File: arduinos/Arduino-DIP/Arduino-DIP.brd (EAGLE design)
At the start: 23.5 x 57.3 mm, 16 parts, among them IC1 ATMEGA 328, IC2 MCP1702-33, X1 16 MHz

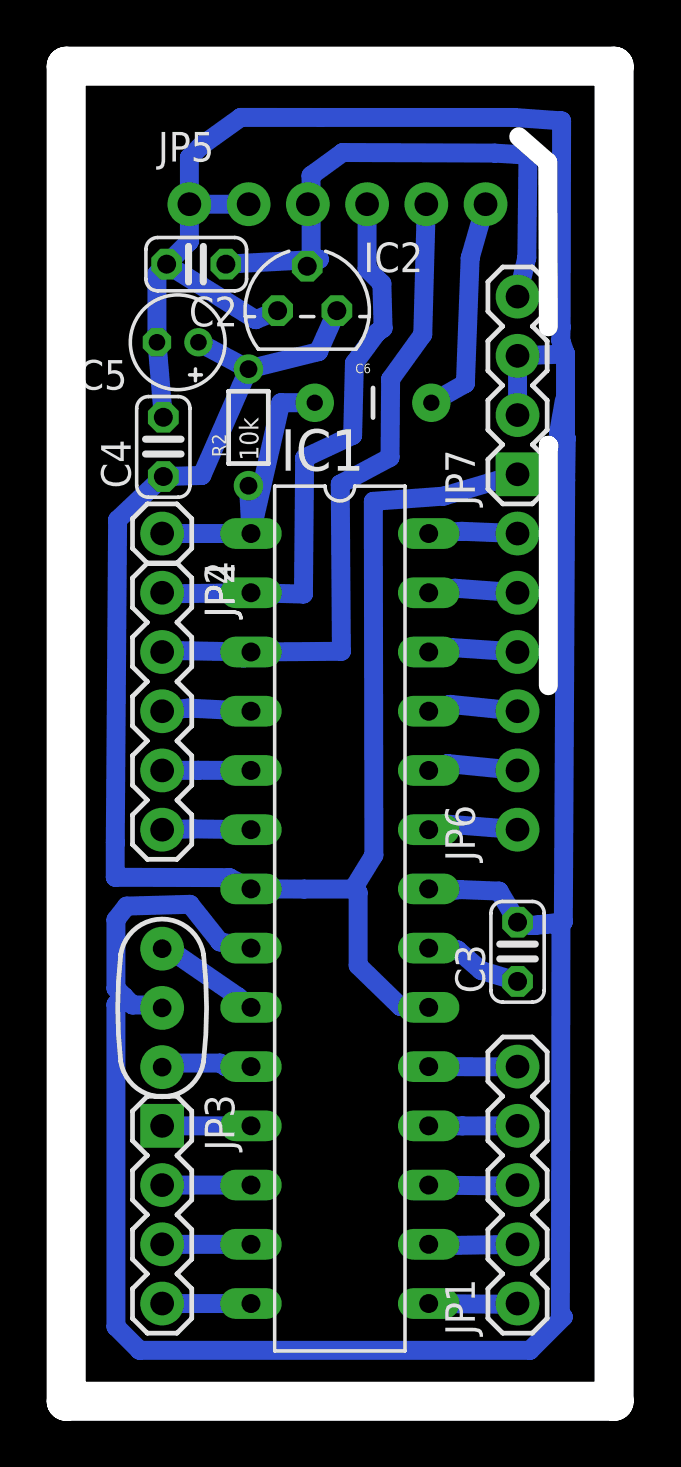
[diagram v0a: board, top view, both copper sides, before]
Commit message: much commit, so wow
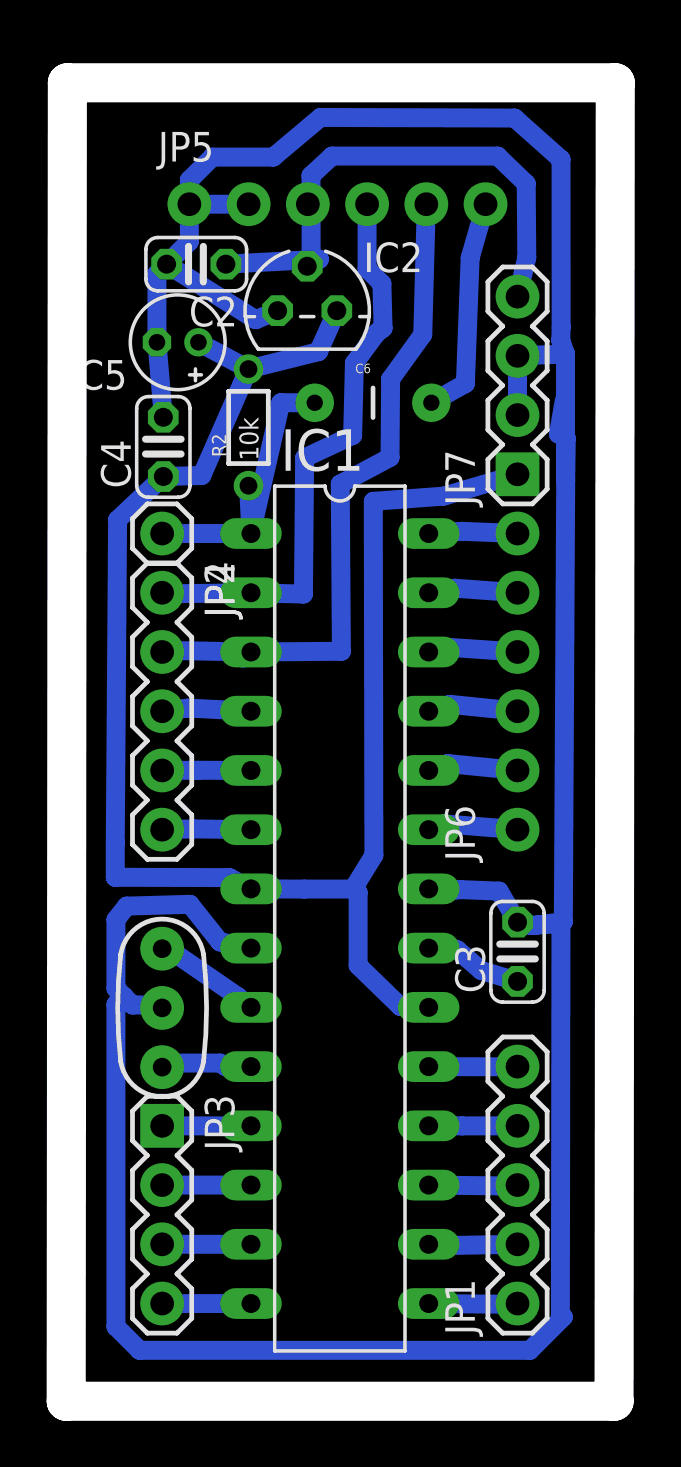
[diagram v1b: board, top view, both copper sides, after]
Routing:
- net GND: track 150.5 -> 149.0 mm
- net PWR: track 24.3 -> 23.5 mm
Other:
- board size 23.5 x 57.3 mm -> 23.5 x 56.5 mm
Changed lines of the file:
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@@
 <layer number="21" name="tPlace" color="7" fill="1" visible="yes" active="yes"/>
 <layer number="22" name="bPlace" color="7" fill="1" visible="yes" active="yes"/>
-<layer number="23" name="tOrigins" color="15" fill="1" visible="yes" active="yes"/>
-<layer number="24" name="bOrigins" color="15" fill="1" visible="yes" active="yes"/>
+<layer number="23" name="tOrigins" color="15" fill="1" visible="no" active="yes"/>
+<layer number="24" name="bOrigins" color="15" fill="1" visible="no" active="yes"/>
 <layer number="25" name="tNames" color="7" fill="1" visible="no" active="yes"/>
 <layer number="26" name="bNames" color="7" fill="1" visible="no" active="yes"/>
@@
 <layer number="112" name="tSilk" color="7" fill="1" visible="yes" active="yes"/>
 <layer number="113" name="IDFDebug" color="4" fill="1" visible="yes" active="yes"/>
-<layer number="114" name="roland_bottom_32" color="11" fill="1" visible="yes" active="yes"/>
+<layer number="114" name="roland_bottom_32" color="11" fill="1" visible="no" active="yes"/>
 <layer number="116" name="Patch_BOT" color="9" fill="4" visible="yes" active="yes"/>
 <layer number="121" name="_tsilk" color="7" fill="1" visible="yes" active="yes"/>
@@
 A0</text>
 <wire x1="0" y1="0" x2="23.495" y2="0" width="1.6764" layer="20"/>
-<wire x1="23.495" y1="0" x2="23.495" y2="57.2516" width="1.6764" layer="20"/>
-<wire x1="23.495" y1="57.2516" x2="0" y2="57.2516" width="1.6764" layer="20"/>
-<wire x1="0" y1="57.2516" x2="0" y2="0" width="1.6764" layer="20"/>
+<wire x1="23.495" y1="0" x2="23.5458" y2="56.5404" width="1.6764" layer="20"/>
+<wire x1="23.5458" y1="56.5404" x2="0.0508" y2="56.5404" width="1.6764" layer="20"/>
+<wire x1="0.0508" y1="56.5404" x2="0" y2="0" width="1.6764" layer="20"/>
 <wire x1="14.3002" y1="2.9718" x2="9.271" y2="2.9718" width="0.8128" layer="114"/>
-<wire x1="19.4056" y1="54.229" x2="20.6502" y2="53.1368" width="0.8128" layer="46"/>
-<wire x1="20.6502" y1="53.1368" x2="20.6756" y2="46.0756" width="0.8128" layer="46"/>
-<wire x1="20.701" y1="40.9702" x2="20.6756" y2="40.9956" width="0.8128" layer="46"/>
-<wire x1="20.6756" y1="40.9956" x2="20.6756" y2="30.6832" width="0.8128" layer="46"/>
+<wire x1="19.4056" y1="54.229" x2="20.6502" y2="53.1368" width="0.8128" layer="114"/>
+<wire x1="20.6502" y1="53.1368" x2="20.6756" y2="46.0756" width="0.8128" layer="114"/>
+<wire x1="20.701" y1="40.9702" x2="20.6756" y2="40.9956" width="0.8128" layer="114"/>
+<wire x1="20.6756" y1="40.9956" x2="20.6756" y2="30.6832" width="0.8128" layer="114"/>
 </plain>
 <attributes>
@@
 <wire x1="19.44059375" y1="20.4738" x2="19.3548" y2="20.5440125" width="0.8128" layer="16"/>
 <wire x1="21.2174" y1="20.493" x2="19.9524" y2="20.3992" width="0.8128" layer="16"/>
-<wire x1="21.2448" y1="54.907" x2="19.2048" y2="55.0532" width="0.8128" layer="16"/>
-<wire x1="19.2048" y1="55.0532" x2="10.9048" y2="55.0532" width="0.8128" layer="16"/>
-<wire x1="10.9048" y1="55.0532" x2="7.4856" y2="55.0548" width="0.8128" layer="16"/>
-<wire x1="7.4856" y1="55.0548" x2="5.784" y2="53.835428125" width="0.8128" layer="16"/>
-<wire x1="21.2448" y1="54.907" x2="21.225290625" y2="46.05624375" width="0.8128" layer="16"/>
+<wire x1="21.2194" y1="53.256" x2="19.2302" y2="55.0278" width="0.8128" layer="16"/>
+<wire x1="19.2302" y1="55.0278" x2="10.9048" y2="55.0532" width="0.8128" layer="16"/>
+<wire x1="10.9048" y1="55.0532" x2="8.8826" y2="53.353" width="0.8128" layer="16"/>
+<wire x1="8.8826" y1="53.353" x2="6.2666" y2="53.352828125" width="0.8128" layer="16"/>
+<wire x1="21.2194" y1="53.256" x2="21.225290625" y2="46.05624375" width="0.8128" layer="16"/>
 <wire x1="21.319" y1="20.561" x2="21.4206" y2="39.497" width="0.8128" layer="16"/>
 <wire x1="21.4206" y1="39.497" x2="21.446" y2="41.292" width="0.8128" layer="16"/>
@@
 <contactref element="JP5" pad="1"/>
 <contactref element="JP5" pad="2"/>
-<wire x1="5.2832" y1="51.3334" x2="5.2832" y2="53.334628125" width="0.8128" layer="16"/>
-<wire x1="5.2832" y1="53.334628125" x2="5.784" y2="53.835428125" width="0.8128" layer="16"/>
+<wire x1="5.2832" y1="51.3334" x2="5.2832" y2="52.369428125" width="0.8128" layer="16"/>
+<wire x1="5.2832" y1="52.369428125" x2="6.2666" y2="53.352828125" width="0.8128" layer="16"/>
 <wire x1="7.8232" y1="51.3334" x2="5.2832" y2="51.3334" width="0.8128" layer="16"/>
 <wire x1="5.2832" y1="51.3334" x2="5.2832" y2="49.738075" width="0.8128" layer="16"/>
@@
 <contactref element="IC2" pad="2"/>
 <contactref element="C2" pad="1"/>
-<wire x1="19.8032" y1="53.4358" x2="18.3746" y2="53.5246" width="0.8128" layer="16"/>
-<wire x1="18.3746" y1="53.5246" x2="11.8588" y2="53.55" width="0.8128" layer="16"/>
-<wire x1="11.8588" y1="53.55" x2="10.4984" y2="52.561" width="0.8128" layer="16"/>
+<wire x1="19.727" y1="52.2166" x2="18.5016" y2="53.3976" width="0.8128" layer="16"/>
+<wire x1="18.5016" y1="53.3976" x2="11.4016" y2="53.3976" width="0.8128" layer="16"/>
+<wire x1="11.4016" y1="53.3976" x2="10.4984" y2="52.561" width="0.8128" layer="16"/>
 <wire x1="10.4984" y1="52.561" x2="10.5048" y2="51.341028125" width="0.8128" layer="16"/>
 <wire x1="10.858109375" y1="48.971971875" x2="10.3359875" y2="48.6730875" width="0.8128" layer="16"/>
-<wire x1="19.7524" y1="49.0372" x2="19.8032" y2="53.4358" width="0.8128" layer="16"/>
+<wire x1="19.7524" y1="49.0372" x2="19.727" y2="52.2166" width="0.8128" layer="16"/>
 <wire x1="6.846940625" y1="48.761815625" x2="10.858109375" y2="48.971971875" width="0.8128" layer="16"/>
 <contactref element="JP7" pad="4"/>
